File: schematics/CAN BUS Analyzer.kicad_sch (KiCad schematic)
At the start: 2 parts, among them U1 ATSAME51J18A-A, U2 TCAN1043xDxQ1

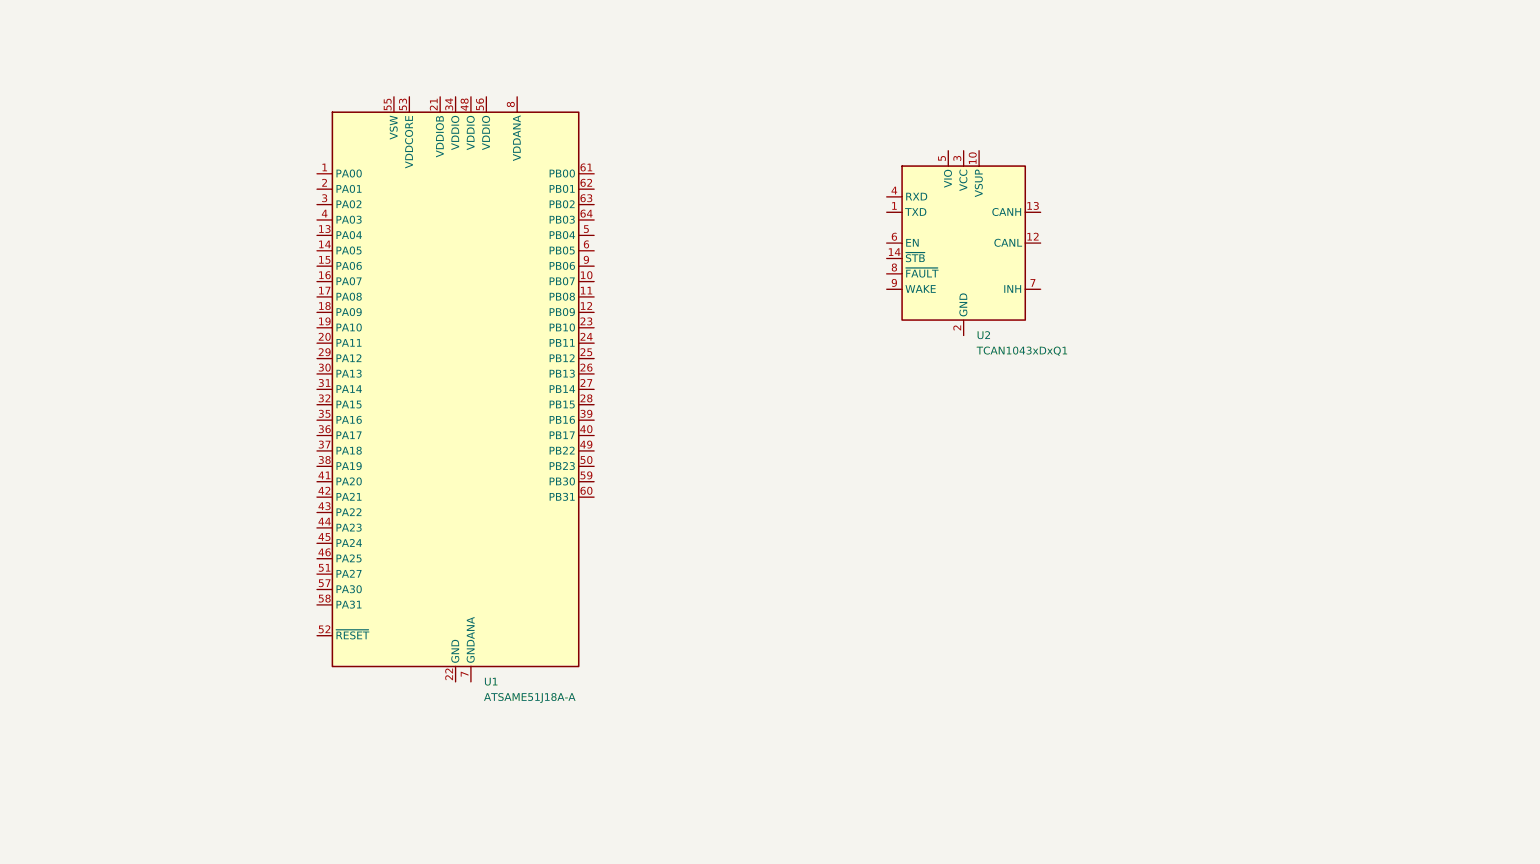
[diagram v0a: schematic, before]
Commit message: smaller changes, cpu and conn
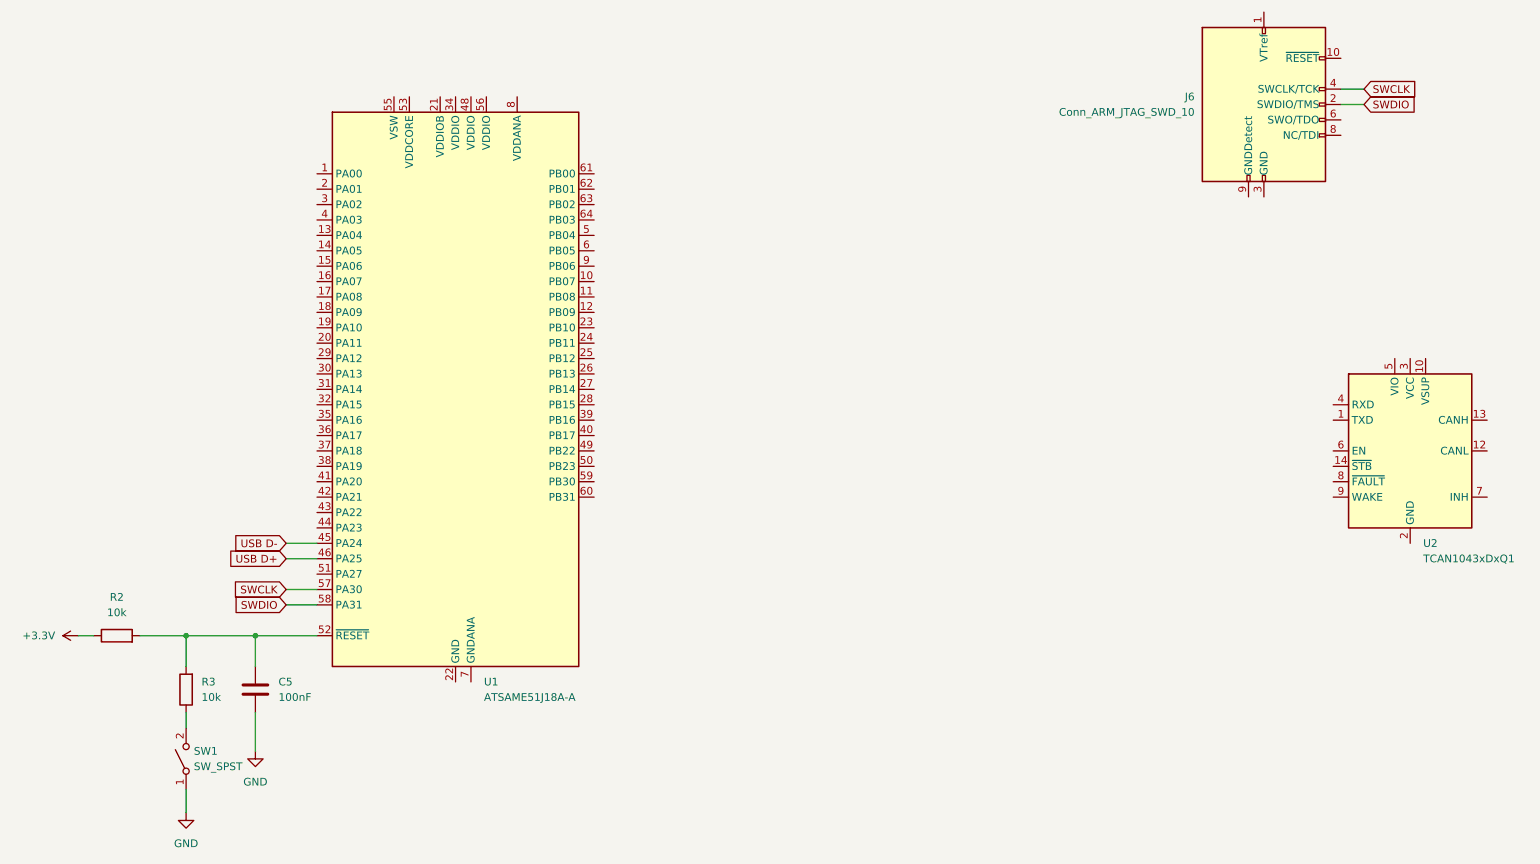
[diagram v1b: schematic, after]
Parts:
- added C5: 100nF, symbol Device:C
- added J6: Conn_ARM_JTAG_SWD_10, Connector_PinHeader_1.27mm:PinHeader_2x05_P1.27mm_Vertical, symbol Connector:Conn_ARM_JTAG_SWD_10
- added R2, R3: 10k, symbol Device:R
- added SW1: SW_SPST, symbol Switch:SW_SPST
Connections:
- net USB D-: now reaches U1.45 (PA24)
- net USB D+: now reaches U1.46 (PA25)
- net at U1.52 (~{RESET}): now also C5.1, R2.2, R3.2
- net SWCLK: now reaches U1.57 (PA30)
- net SWCLK: now also J6.4 (SWCLK/TCK)
- net SWDIO: now reaches U1.58 (PA31)
- net SWDIO: now also J6.2 (SWDIO/TMS)
- new net: J6.3 (GND), J6.5 (GND)
- new net: R3.1, SW1.2 (B)
- new net +3.3V: R2.1
- new net GND: C5.2, SW1.1 (A)
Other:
- moved on the sheet: U2
